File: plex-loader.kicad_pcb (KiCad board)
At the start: 4 copper layers, 38.1 x 68 mm, 48 parts, among them J1 Conn_01x05_Pin, J10 Conn_02x05_Odd_Even, J2 Conn_01x05_Pin, J3 Conn_01x05_Pin, J4 Conn_01x05_Pin, J5 Conn_01x05_Pin, J6 Conn_01x05_Pin, J9 Conn_02x20_Odd_Even, U1 TMUX1208PWR, U2 TMUX1208PWR, U3 TMUX1208PWR, U4 DSPIC33FJ128GP204, U5 SQ3457EV-T1_BE3

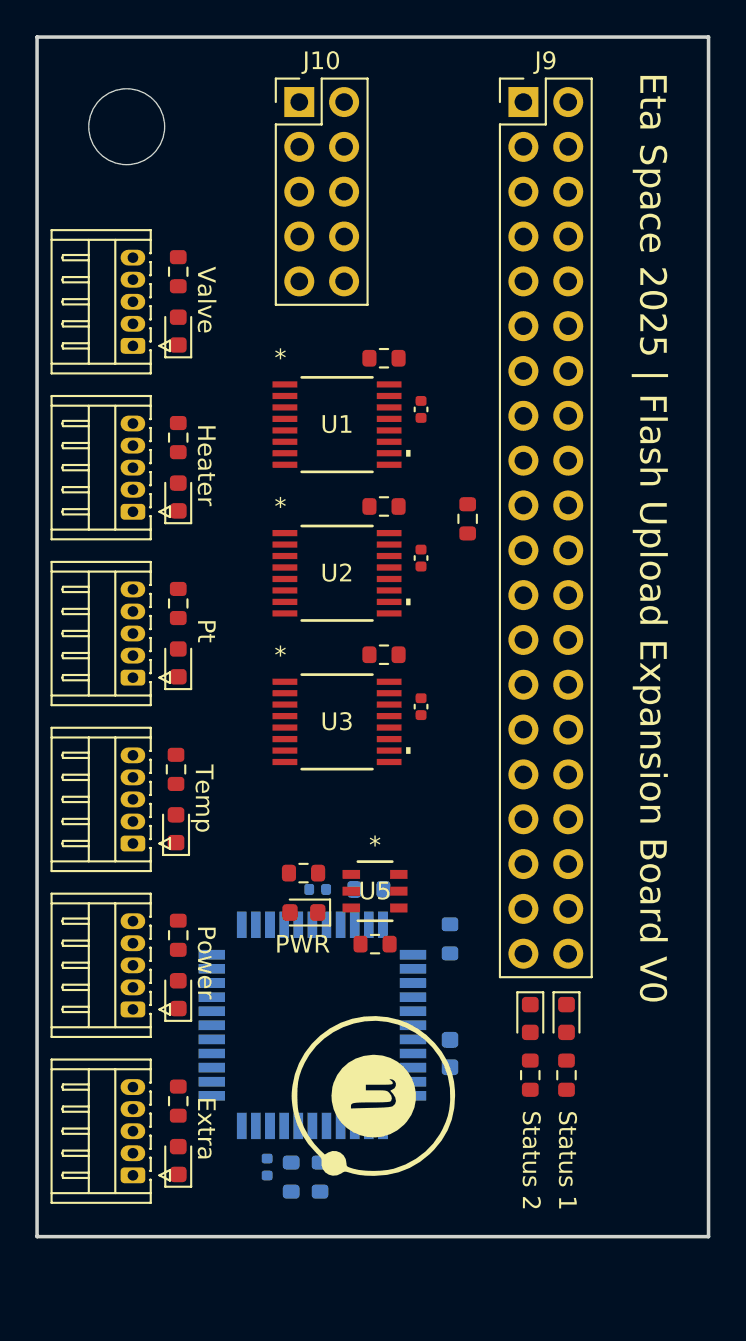
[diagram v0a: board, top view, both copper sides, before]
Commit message: curtis changes
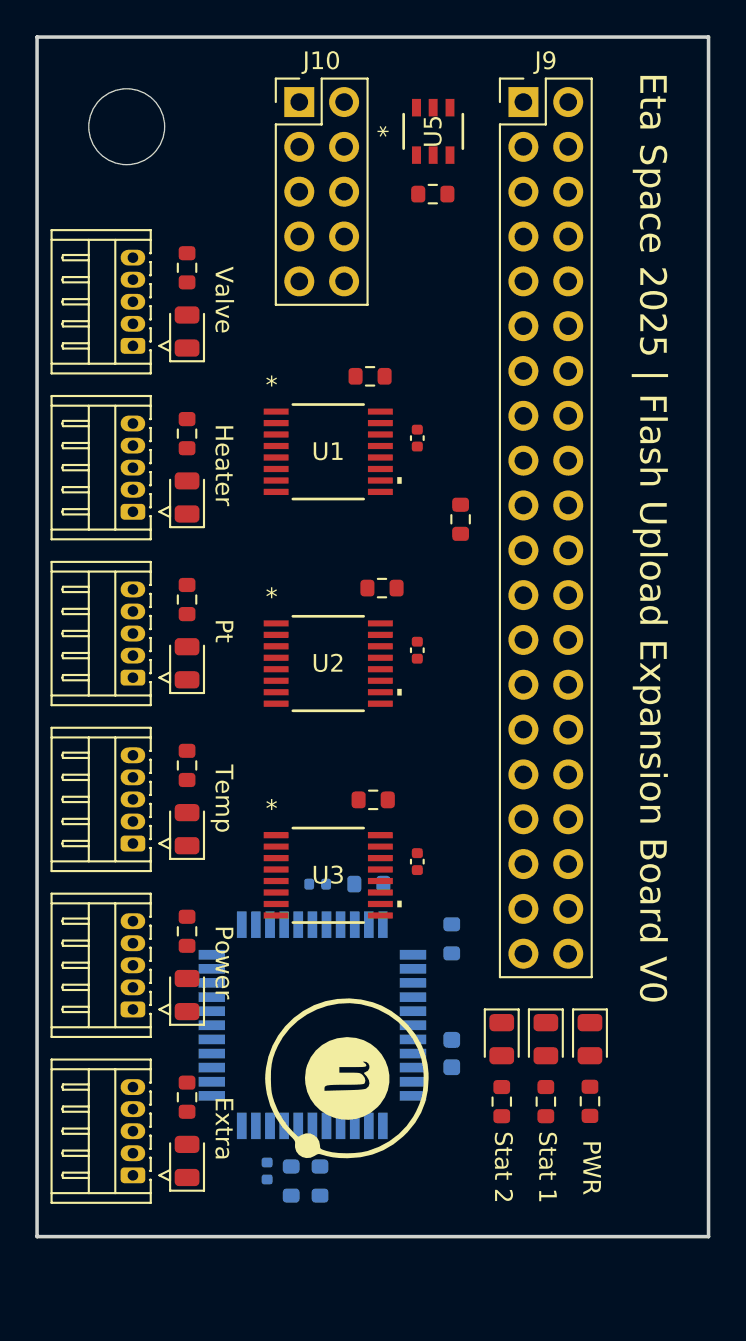
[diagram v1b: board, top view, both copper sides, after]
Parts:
- D1, D2, D3, D4, D5, D6, D7, D8, D9: footprint LED_SMD:LED_0603_1608Metric -> LED_SMD:LED_0805_2012Metric
- R11, R12, R13, R14, R15, R16, R17, R18: value 50 -> 1k
- moved U5 43.2 mm to (72.4, 55.3), turned to 90 degrees
- moved R3 42.6 mm to (72.4, 58.9), turned to 0 degrees
- moved R4 20.8 mm to (81.3, 110.3), turned to 90 degrees
- moved D1 17.7 mm to (81.3, 106.8), turned to -90 degrees
- moved C3 8.78 mm to (71.5, 96.7)
- moved U3 8.71 mm to (66.5, 97.5)
- moved R7 8.25 mm to (69.0, 93.2), turned to 0 degrees
- moved C2 5.23 mm to (71.5, 84.7)
- moved U2 5.14 mm to (66.5, 85.5)
- moved R8 4.63 mm to (69.5, 81.2)
- moved R18 2.21 mm to (76.3, 110.3)
- moved D9 2.00 mm to (76.3, 106.8)
- moved R17 1.90 mm to (78.8, 110.3)
- moved G*** 1.80 mm to (67.5, 109.0)
- moved D8 1.66 mm to (78.8, 106.8)
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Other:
- board text added: "Stat 1"
- board text added: "Stat 2"
- board text removed: "Status 1"
- board text removed: "Status 2"
